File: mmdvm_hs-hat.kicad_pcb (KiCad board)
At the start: 2 copper layers, 65.1 x 30.2 mm, 138 parts, among them P1 BOOT0, P2 DISPLAY, P3 SMA, P4 STLINK, SW1 SW_DIP_x01, U1 ADF7021, U2 STM32F103C8T6, X1 TCXO, Y1 8MHz

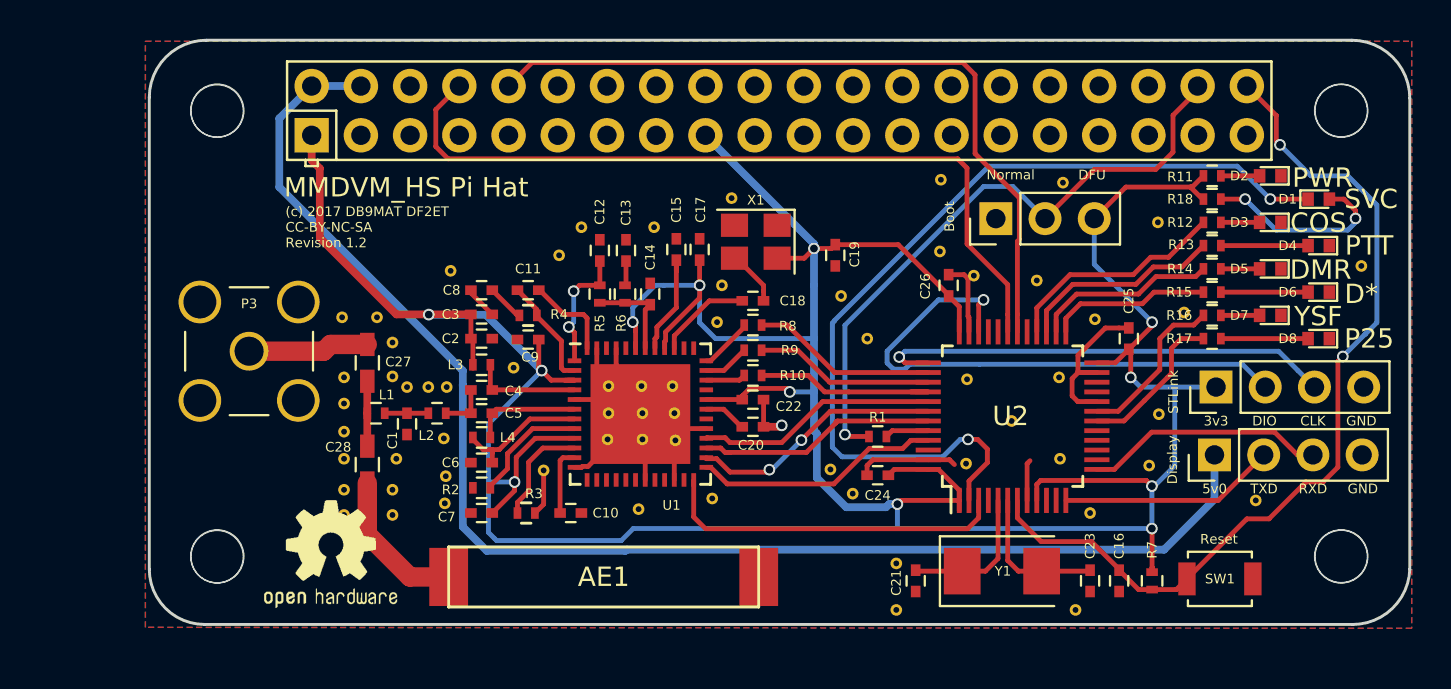
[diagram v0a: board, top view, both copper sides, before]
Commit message: The commit of MMDVM Hat VHF project
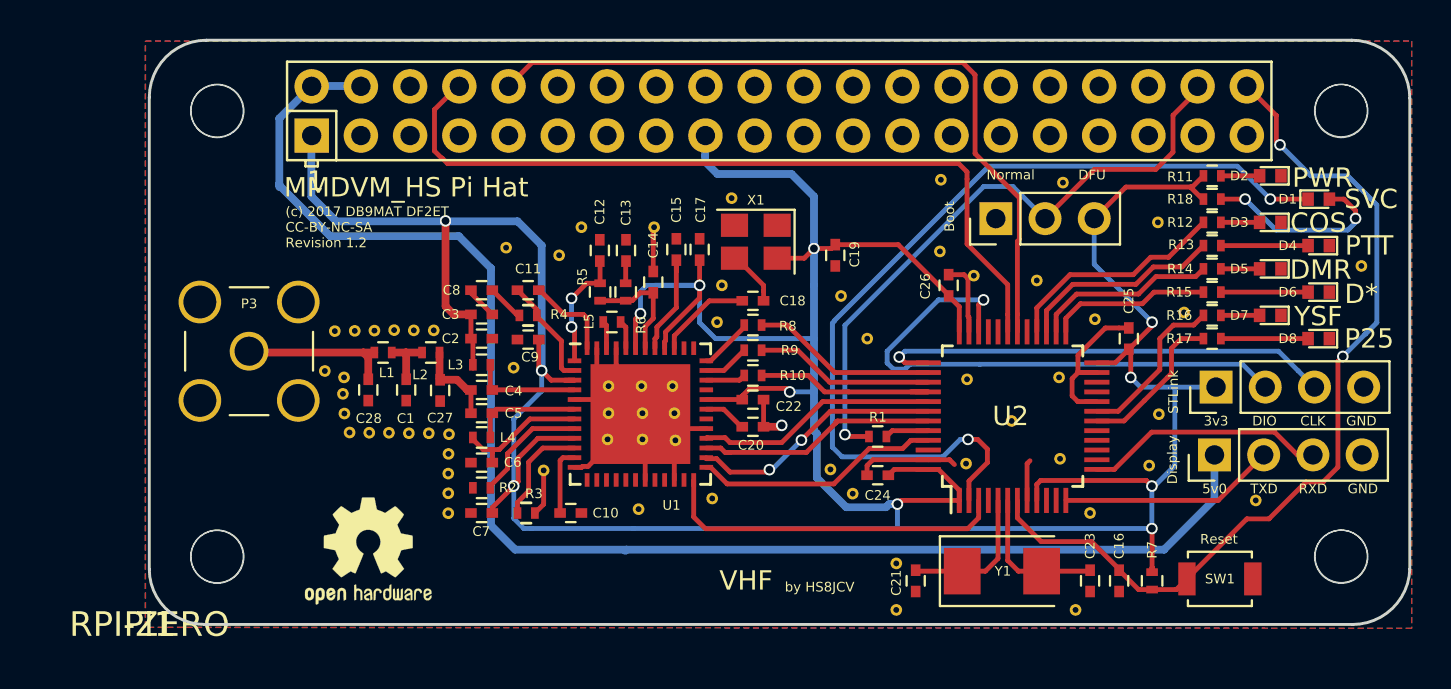
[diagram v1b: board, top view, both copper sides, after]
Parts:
- removed AE1: AN1603_433, MMDVM:AN1603
- removed G***: LOGO, OPENHARDWARE:OSHWLOGO0.3IN
- removed the REF** at (168.0, 130.1)
- removed the REF** at (165.5, 130.1)
- removed the REF** at (170.8, 123.5)
- removed the REF** at (165.5, 125.8)
- removed the REF** at (165.5, 124.3)
- removed the REF** at (168.8, 123.5)
- removed the REF** at (165.4, 119.9)
- removed the REF** at (167.2, 119.9)
- removed the REF** at (165.5, 127.2)
- removed the REF** at (168.2, 127.2)
- removed the REF** at (165.5, 128.8)
- removed the REF** at (169.8, 123.5)
- removed the REF** at (170.7, 126.2)
- removed the REF** at (171.0, 117.5)
- added L5: 20n, Resistors_SMD:R_0402, F.Cu at (179.3, 120.1)
- added REF**: VIA-0.6mm, MMDVM:VIA-0.6mm, F.Cu at (173.9, 116.3)
- added REF**: VIA-0.6mm, MMDVM:VIA-0.6mm, F.Cu at (165.8, 125.8)
- added REF**: VIA-0.6mm, MMDVM:VIA-0.6mm, F.Cu at (166.8, 125.9)
- added REF**: VIA-0.6mm, MMDVM:VIA-0.6mm, F.Cu at (167.8, 125.9)
- added REF**: VIA-0.6mm, MMDVM:VIA-0.6mm, F.Cu at (169.9, 125.9)
- added REF**: VIA-0.6mm, MMDVM:VIA-0.6mm, F.Cu at (170.9, 125.9)
- added REF**: VIA-0.6mm, MMDVM:VIA-0.6mm, F.Cu at (170.9, 126.9)
- added REF**: VIA-0.6mm, MMDVM:VIA-0.6mm, F.Cu at (170.9, 128.0)
- added REF**: VIA-0.6mm, MMDVM:VIA-0.6mm, F.Cu at (164.5, 122.7)
- added REF**: VIA-0.6mm, MMDVM:VIA-0.6mm, F.Cu at (170.1, 120.6)
- added REF**: VIA-0.6mm, MMDVM:VIA-0.6mm, F.Cu at (165.0, 120.6)
- added REF**: VIA-0.6mm, MMDVM:VIA-0.6mm, F.Cu at (166.1, 120.6)
- added REF**: VIA-0.6mm, MMDVM:VIA-0.6mm, F.Cu at (167.1, 120.6)
- added REF**: VIA-0.6mm, MMDVM:VIA-0.6mm, F.Cu at (168.1, 120.6)
- added REF**: VIA-0.6mm, MMDVM:VIA-0.6mm, F.Cu at (169.1, 120.6)
- added REF**: VIA-0.6mm, MMDVM:VIA-0.6mm, F.Cu at (165.4, 123.9)
- added REF**: VIA-0.6mm, MMDVM:VIA-0.6mm, F.Cu at (165.5, 124.9)
- added REF***: OSHW-Logo2_7.3x6mm_SilkScreen, Symbols:OSHW-Logo2_7.3x6mm_SilkScreen, F.Cu at (166.8, 132.0)
- C1: value 6p8 -> 15p
- C12: value 470p -> 82p
- C13: value 15n -> 2.7n
- C14: value 1n -> 200p
- C27, C28: value 100n -> 15p; footprint Capacitors_SMD:C_0603_HandSoldering -> Capacitors_SMD:C_0402
- C4: value 10p -> 18p
- C5: value 4p7 -> 12p
- C6: value 6p8 -> 10p
- L1: value 22n -> 150n
- L2: value 20n -> 130n
- L3: value 13n -> 100n
- L4: value 27n -> 200n
- R3: value 3k8 -> 3k6
- R4: value 3r9 -> 2r
- R5: value 560 -> 3.4K
- R6: value 270 -> 1.65K
- moved C27 4.02 mm to (170.5, 123.7)
- moved C28 3.85 mm to (166.8, 123.6)
- moved L1 3.15 mm to (167.5, 121.7)
- moved L2 3.15 mm to (170.0, 121.7)
- moved REF** 3.04 mm to (168.8, 125.9)
- moved C1 1.75 mm to (168.7, 123.6)
- moved REF** 0.89 mm to (170.9, 129.0)
- moved C14 0.64 mm to (181.5, 118.1)
- moved REF** 0.54 mm to (170.9, 130.0)
- moved R6 0.11 mm to (180.0, 118.6)
- moved R5 0.11 mm to (178.7, 118.6)
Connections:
- C27 pad 2: RF -> GND
- C28 pad 1: RF -> Net-(C28-Pad1)
- C28 pad 2: Net-(AE1-Pad1) -> GND
- C4 pad 2: Net-(C4-Pad2) -> Net-(C27-Pad1)
- C5 pad 2: Net-(C4-Pad2) -> Net-(C27-Pad1)
- L1 pad 1: RF -> Net-(C28-Pad1)
- L2 pad 2: Net-(C4-Pad2) -> Net-(C27-Pad1)
- P3 pad 1: Net-(C27-Pad1) -> Net-(C28-Pad1)
- PI1 pad 11: (no net) -> Net-(PI1-Pad11)
- PI1 pad 12: (no net) -> Net-(PI1-Pad12)
- PI1 pad 13: (no net) -> Net-(PI1-Pad13)
- PI1 pad 15: (no net) -> Net-(PI1-Pad15)
- PI1 pad 16: (no net) -> Net-(PI1-Pad16)
- PI1 pad 18: (no net) -> Net-(PI1-Pad18)
- PI1 pad 19: (no net) -> Net-(PI1-Pad19)
- PI1 pad 21: (no net) -> Net-(PI1-Pad21)
- PI1 pad 22: (no net) -> Net-(PI1-Pad22)
- PI1 pad 24: (no net) -> Net-(PI1-Pad24)
- PI1 pad 26: (no net) -> Net-(PI1-Pad26)
- PI1 pad 27: (no net) -> Net-(PI1-Pad27)
- PI1 pad 28: (no net) -> Net-(PI1-Pad28)
- PI1 pad 29: (no net) -> Net-(PI1-Pad29)
- PI1 pad 3: (no net) -> Net-(PI1-Pad3)
- PI1 pad 31: (no net) -> Net-(PI1-Pad31)
- PI1 pad 32: (no net) -> Net-(PI1-Pad32)
- PI1 pad 33: (no net) -> Net-(PI1-Pad33)
- PI1 pad 35: (no net) -> Net-(PI1-Pad35)
- PI1 pad 36: (no net) -> Net-(PI1-Pad36)
- PI1 pad 5: (no net) -> Net-(PI1-Pad5)
- PI1 pad 7: (no net) -> Net-(PI1-Pad7)
- U1 pad 13: (no net) -> Net-(U1-Pad13)
- U1 pad 14: (no net) -> Net-(U1-Pad14)
- U1 pad 15: (no net) -> Net-(U1-Pad15)
- U1 pad 16: (no net) -> Net-(U1-Pad16)
- U1 pad 17: (no net) -> Net-(U1-Pad17)
- U1 pad 18: (no net) -> Net-(U1-Pad18)
- U1 pad 20: (no net) -> Net-(U1-Pad20)
- U1 pad 21: (no net) -> Net-(U1-Pad21)
- U1 pad 23: (no net) -> Net-(U1-Pad23)
- U1 pad 30: (no net) -> Net-(U1-Pad30)
- U1 pad 33: (no net) -> Net-(U1-Pad33)
- U1 pad 37: (no net) -> Net-(U1-Pad37)
- U1 pad 38: (no net) -> Net-(U1-Pad38)
- U1 pad 44: (no net) -> Net-(L5-Pad2)
- U1 pad 46: (no net) -> Net-(L5-Pad1)
- U2 pad 10: (no net) -> Net-(U2-Pad10)
- U2 pad 11: (no net) -> Net-(U2-Pad11)
- U2 pad 14: (no net) -> Net-(U2-Pad14)
- U2 pad 15: (no net) -> Net-(U2-Pad15)
- U2 pad 16: (no net) -> Net-(U2-Pad16)
- U2 pad 17: (no net) -> Net-(U2-Pad17)
- U2 pad 21: (no net) -> SDA
- U2 pad 22: (no net) -> SCL
- U2 pad 29: (no net) -> Net-(U2-Pad29)
- U2 pad 32: (no net) -> Net-(U2-Pad32)
- U2 pad 33: (no net) -> Net-(U2-Pad33)
- U2 pad 4: (no net) -> Net-(U2-Pad4)
- U2 pad 46: (no net) -> Net-(U2-Pad46)
- X1 pad 1: (no net) -> Net-(X1-Pad1)
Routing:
- net Net-(C28-Pad1): track 0.00 -> 7.98 mm
- net Net-(AE1-Pad1): track 7.76 -> 0.00 mm
- net +3V3: track 195.0 -> 202.3 mm
- net RF: track 3.35 -> 0.00 mm
- net +5V: track 72.6 -> 75.8 mm
- net GND: track 37.7 -> 40.8 mm
- net Net-(C4-Pad2): track 2.50 -> 0.00 mm
- net Net-(C27-Pad1): track 6.24 -> 4.43 mm
- net Net-(L5-Pad2): track 0.00 -> 1.46 mm
- net Net-(L5-Pad1): track 0.00 -> 1.42 mm
- net Net-(C14-Pad1): track 4.99 -> 5.94 mm
- net Net-(C1-Pad1): track 2.25 -> 2.97 mm
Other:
- board text added: "VHF"
- board text added: "by HS8JCV"
